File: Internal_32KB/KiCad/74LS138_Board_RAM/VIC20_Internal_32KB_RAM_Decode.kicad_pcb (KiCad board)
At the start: 2 copper layers, 12 x 24 mm, 2 parts, among them J1 Signals

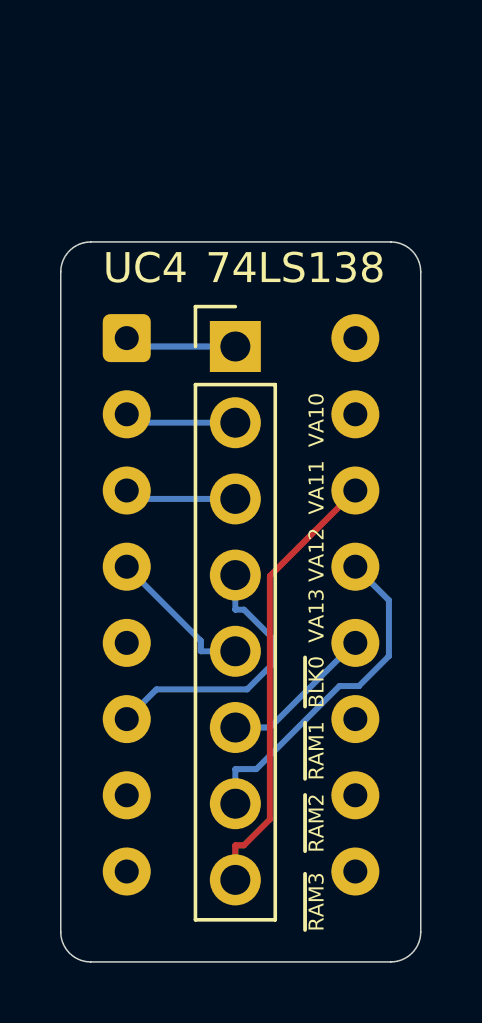
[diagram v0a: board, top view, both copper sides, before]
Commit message: Updates to 32KB board design
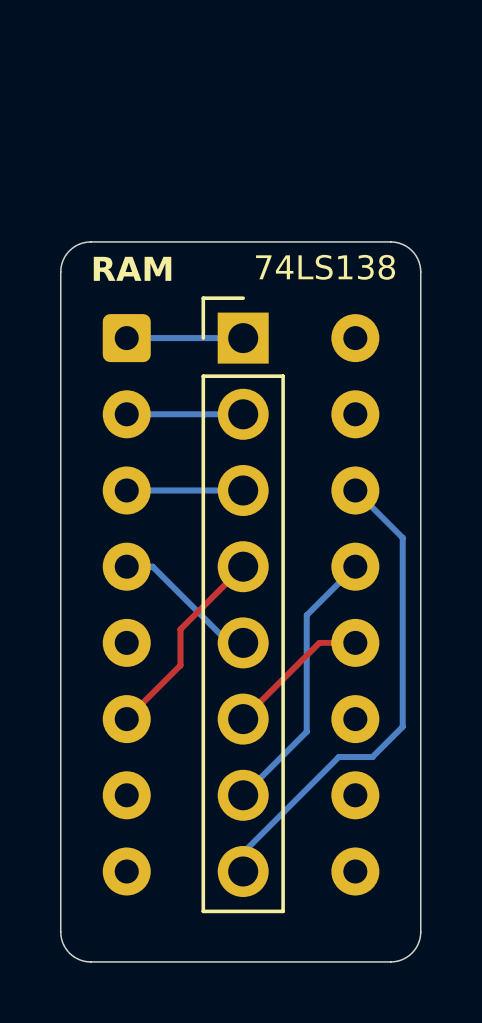
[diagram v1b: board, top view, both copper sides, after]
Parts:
- moved J1 0.38 mm to (76.3, 52.1)
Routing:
- net VA13: track 9.23 -> 6.69 mm
- net ~{RAM2}: track 11.3 -> 9.17 mm
- net ~{RAM3}: track 14.8 -> 16.2 mm
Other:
- board text added: "RAM"
- board text added: "VIC-20 RAM Decoder Logic Replacement Brett Hallen, May 2025"
- board text removed: "VIC-20 Internal 8KB RAM Brett Hallen, May 2025"
- board text removed: "~{RAM3} ~{RAM2} ~{RAM1} ~{BLK0} VA13 VA12 VA11 VA10"
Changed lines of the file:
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@@
 		(allow_soldermask_bridges_in_footprints no)
 		(tenting front back)
+		(grid_origin 72.38 52.1)
 		(pcbplotparams
 			(layerselection 0x00000000_00000000_55555555_5755f5ff)
@@
 	(footprint "Connector_PinHeader_2.54mm:PinHeader_1x08_P2.54mm_Vertical"
 		(layer "F.Cu")
-		(at 76 52.38)
+		(at 76.261842 52.1)
 		(descr "Through hole straight pin header, 1x08, 2.54mm pitch, single row")
 		(tags "Through hole pin header THT 1x08 2.54mm single row")
@@
 		(tags "THT DIP DIL PDIP 2.54mm 7.62mm 300mil")
 		(property "Reference" "UC4"
-			(at 0.62 -2.33 0)
+			(at -0.38 -2.33 0)
 			(layer "F.SilkS")
-			(effects
-				(font
-					(size 1 1)
+			(hide yes)
+			(effects
+				(font
+					(size 0.8 0.8)
 					(thickness 0.15)
 				)
@@
 		)
 		(property "Value" "74LS138"
-			(at 5.62 -2.33 0)
+			(at 6.62 -2.33 0)
 			(layer "F.SilkS")
 			(effects
 				(font
-					(size 1 1)
+					(size 0.8 0.8)
 					(thickness 0.15)
 				)
@@
 		(layer "Edge.Cuts")
 	)
-	(gr_text "~{RAM3}   ~{RAM2}  ~{RAM1}  ~{BLK0}  VA13 VA12  VA11  VA10"
-		(at 79 71.88 90)
+	(gr_text "RAM"
+		(at 71.1801 50.28875 0)
 		(layer "F.SilkS")
 		(effects
 			(font
-				(size 0.5 0.5)
-				(thickness 0.125)
+				(size 0.8 0.8)
+				(thickness 0.15)
+				(bold yes)
 			)
 			(justify left bottom)
 		)
 	)
-	(gr_text "VIC-20 Internal 8KB RAM\nBrett Hallen, May 2025"
-		(at 77.27 70.476051 270)
+	(gr_text "VIC-20 RAM Decoder Logic Replacement\n\n\n\n\nBrett Hallen, May 2025"
+		(at 74.035939 70.315934 270)
 		(layer "B.SilkS")
 		(effects
@@
 	)
 	(segment
-		(start 76 54.92)
-		(end 72.66 54.92)
+		(start 72.38 54.64)
+		(end 76.261842 54.64)
 		(width 0.2)
 		(layer "B.Cu")
@@
 	)
 	(segment
-		(start 72.66 54.92)
-		(end 72.38 54.64)
-		(width 0.2)
-		(layer "B.Cu")
-		(net 1)
-	)
-	(segment
-		(start 76.6983 66.4683)
-		(end 76 66.4683)
+		(start 78.38 65.221842)
+		(end 78.38 61.34)
 		(width 0.2)
 		(layer "B.Cu")
@@
 	)
 	(segment
-		(start 81.1176 62.7023)
-		(end 80.1216 63.6983)
+		(start 78.38 61.34)
+		(end 80 59.72)
 		(width 0.2)
 		(layer "B.Cu")
@@
 	)
 	(segment
-		(start 80 59.72)
-		(end 81.1176 60.8376)
+		(start 76.261842 67.34)
+		(end 78.38 65.221842)
 		(width 0.2)
 		(layer "B.Cu")
@@
 	)
 	(segment
-		(start 80.1216 63.6983)
-		(end 79.4683 63.6983)
-		(width 0.2)
-		(layer "B.Cu")
-		(net 2)
-	)
-	(segment
-		(start 76 67.62)
-		(end 76 66.4683)
-		(width 0.2)
-		(layer "B.Cu")
-		(net 2)
-	)
-	(segment
-		(start 79.4683 63.6983)
-		(end 76.6983 66.4683)
-		(width 0.2)
-		(layer "B.Cu")
-		(net 2)
-	)
-	(segment
-		(start 81.1176 60.8376)
-		(end 81.1176 62.7023)
-		(width 0.2)
-		(layer "B.Cu")
-		(net 2)
-	)
-	(segment
-		(start 77.1517 68.1446)
-		(end 77.1517 60.0283)
+		(start 80 57.18)
+		(end 81.579015 58.759015)
+		(width 0.2)
+		(layer "B.Cu")
+		(net 3)
+	)
+	(segment
+		(start 76.261842 69.251255)
+		(end 76.261842 69.88)
+		(width 0.2)
+		(layer "B.Cu")
+		(net 3)
+	)
+	(segment
+		(start 81.579015 65.058695)
+		(end 80.573773 66.063937)
+		(width 0.2)
+		(layer "B.Cu")
+		(net 3)
+	)
+	(segment
+		(start 80.573773 66.063937)
+		(end 79.44916 66.063937)
+		(width 0.2)
+		(layer "B.Cu")
+		(net 3)
+	)
+	(segment
+		(start 79.44916 66.063937)
+		(end 76.261842 69.251255)
+		(width 0.2)
+		(layer "B.Cu")
+		(net 3)
+	)
+	(segment
+		(start 81.579015 58.759015)
+		(end 81.579015 65.058695)
+		(width 0.2)
+		(layer "B.Cu")
+		(net 3)
+	)
+	(segment
+		(start 72.38 57.18)
+		(end 76.261842 57.18)
+		(width 0.2)
+		(layer "B.Cu")
+		(net 4)
+	)
+	(segment
+		(start 73.245617 59.72)
+		(end 75.785617 62.26)
+		(width 0.2)
+		(layer "B.Cu")
+		(net 5)
+	)
+	(segment
+		(start 75.785617 62.26)
+		(end 76.261842 62.26)
+		(width 0.2)
+		(layer "B.Cu")
+		(net 5)
+	)
+	(segment
+		(start 72.38 59.72)
+		(end 73.245617 59.72)
+		(width 0.2)
+		(layer "B.Cu")
+		(net 5)
+	)
+	(segment
+		(start 76.261842 59.72)
+		(end 74.170141 61.811701)
 		(width 0.2)
 		(layer "F.Cu")
-		(net 3)
-	)
-	(segment
-		(start 76 70.16)
-		(end 76 69.0083)
+		(net 6)
+	)
+	(segment
+		(start 74.170141 63.009859)
+		(end 72.38 64.8)
 		(width 0.2)
 		(layer "F.Cu")
-		(net 3)
-	)
-	(segment
-		(start 76 69.0083)
-		(end 76.288 69.0083)
+		(net 6)
+	)
+	(segment
+		(start 74.170141 61.811701)
+		(end 74.170141 63.009859)
 		(width 0.2)
 		(layer "F.Cu")
-		(net 3)
-	)
-	(segment
-		(start 77.1517 60.0283)
-		(end 80 57.18)
+		(net 6)
+	)
+	(segment
+		(start 76.261842 64.8)
+		(end 78.801842 62.26)
 		(width 0.2)
 		(layer "F.Cu")
-		(net 3)
-	)
-	(segment
-		(start 76.288 69.0083)
-		(end 77.1517 68.1446)
+		(net 7)
+	)
+	(segment
+		(start 78.801842 62.26)
+		(end 80 62.26)
 		(width 0.2)
 		(layer "F.Cu")
-		(net 3)
-	)
-	(segment
-		(start 76 57.46)
-		(end 72.66 57.46)
-		(width 0.2)
-		(layer "B.Cu")
-		(net 4)
-	)
-	(segment
-		(start 72.66 57.46)
-		(end 72.38 57.18)
-		(width 0.2)
-		(layer "B.Cu")
-		(net 4)
-	)
-	(segment
-		(start 74.8483 62.54)
-		(end 74.8483 62.1883)
-		(width 0.2)
-		(layer "B.Cu")
-		(net 5)
-	)
-	(segment
-		(start 74.8483 62.1883)
-		(end 72.38 59.72)
-		(width 0.2)
-		(layer "B.Cu")
-		(net 5)
-	)
-	(segment
-		(start 76 62.54)
-		(end 74.8483 62.54)
-		(width 0.2)
-		(layer "B.Cu")
-		(net 5)
-	)
-	(segment
-		(start 76.2879 61.1517)
-		(end 77.1925 62.0563)
-		(width 0.2)
-		(layer "B.Cu")
-		(net 6)
-	)
-	(segment
-		(start 76 61.1517)
-		(end 76.2879 61.1517)
-		(width 0.2)
-		(layer "B.Cu")
-		(net 6)
-	)
-	(segment
-		(start 76.3953 63.81)
-		(end 73.37 63.81)
-		(width 0.2)
-		(layer "B.Cu")
-		(net 6)
-	)
-	(segment
-		(start 77.1925 62.0563)
-		(end 77.1925 63.0128)
-		(width 0.2)
-		(layer "B.Cu")
-		(net 6)
-	)
-	(segment
-		(start 76 60)
-		(end 76 61.1517)
-		(width 0.2)
-		(layer "B.Cu")
-		(net 6)
-	)
-	(segment
-		(start 73.37 63.81)
-		(end 72.38 64.8)
-		(width 0.2)
-		(layer "B.Cu")
-		(net 6)
-	)
-	(segment
-		(start 77.1925 63.0128)
-		(end 76.3953 63.81)
-		(width 0.2)
-		(layer "B.Cu")
-		(net 6)
-	)
-	(segment
-		(start 77.1517 65.08)
-		(end 79.9717 62.26)
-		(width 0.2)
-		(layer "B.Cu")
 		(net 7)
 	)
 	(segment
-		(start 76 65.08)
-		(end 77.1517 65.08)
-		(width 0.2)
-		(layer "B.Cu")
-		(net 7)
-	)
-	(segment
-		(start 79.9717 62.26)
-		(end 80 62.26)
-		(width 0.2)
-		(layer "B.Cu")
-		(net 7)
-	)
-	(segment
-		(start 72.66 52.38)
-		(end 72.38 52.1)
-		(width 0.2)
-		(layer "B.Cu")
-		(net 8)
-	)
-	(segment
-		(start 76 52.38)
-		(end 72.66 52.38)
-		(width 0.2)
-		(layer "B.Cu")
+		(start 72.38 52.1)
+		(end 76.261842 52.1)
+		(width 0.2)
+		(layer "B.Cu")
